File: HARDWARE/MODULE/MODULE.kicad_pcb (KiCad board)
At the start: 4 copper layers, 160 x 100 mm, 119 parts, among them J201 Conn_02x08_Odd_Even, J301 Conn_02x06_Odd_Even, Q201 2N7002, Q202 2N7002, Q203 TIP41C/D44H, Q204 MMBT3904, Q205 PZT2907A, Q206 PZT2222A, Q207 MMBT3906, Q208 TIP42C/D45H, U301 LM317_TO-263, U302 LT8330_S6, U303 LM337_TO263, U304 LT8570_MS8E, U305 L78L15_SO8, U306 TEL10-2415, U307 SN6505BDBV, U308 L79L15_SO8

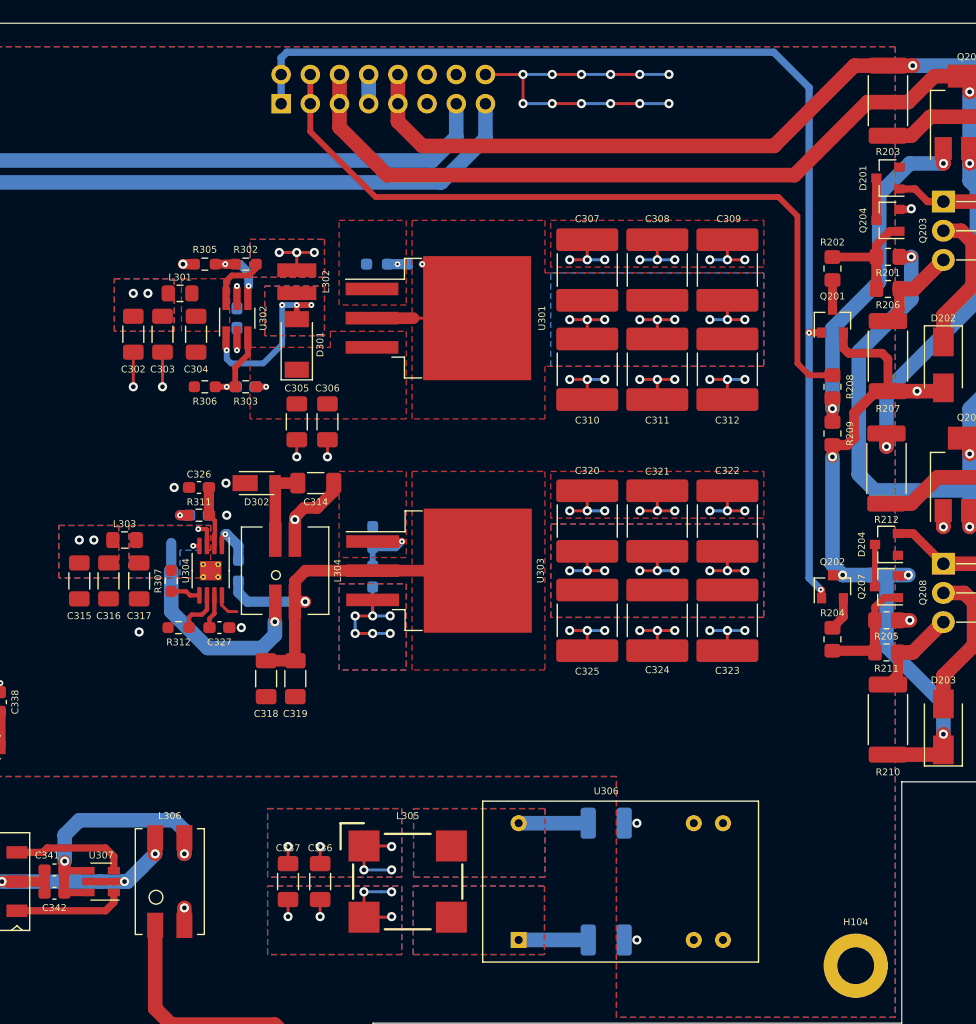
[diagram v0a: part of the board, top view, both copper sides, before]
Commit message: PCB changes
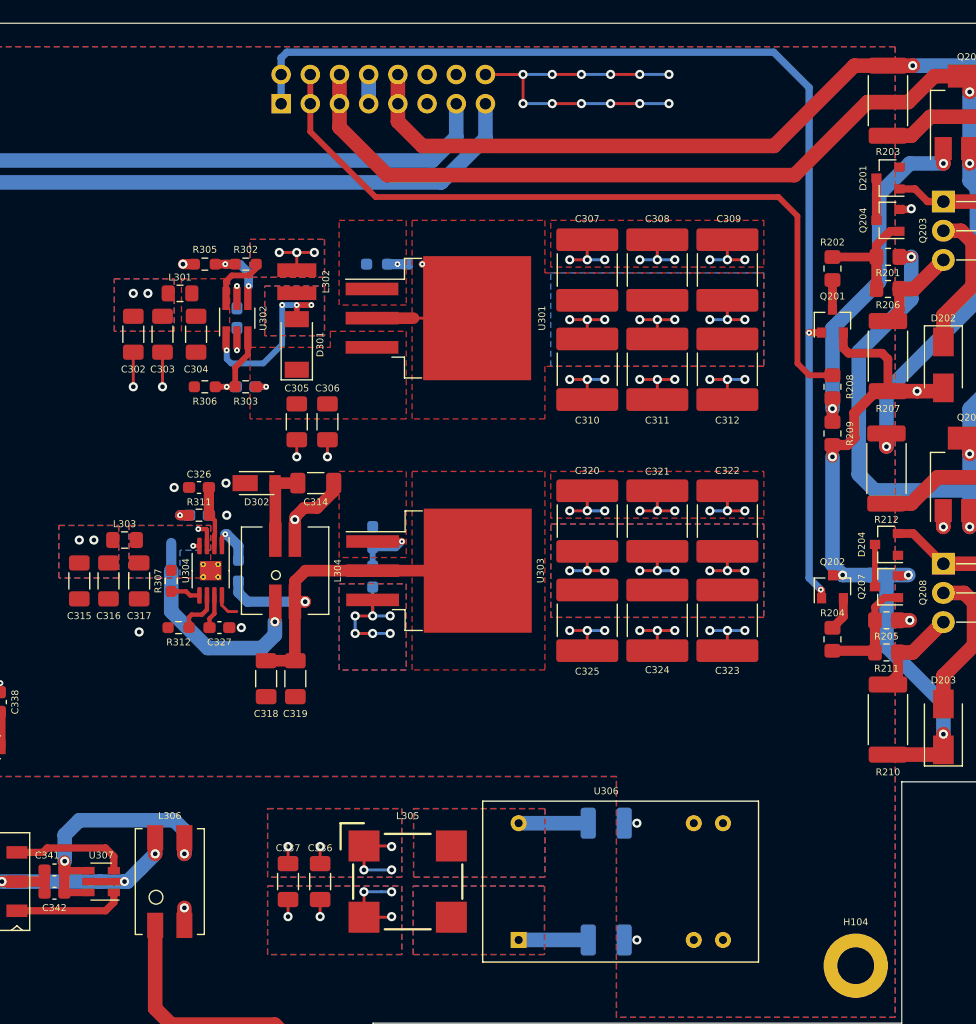
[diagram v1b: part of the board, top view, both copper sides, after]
